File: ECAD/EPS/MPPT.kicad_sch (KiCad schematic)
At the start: 22 parts, among them U13 INA180A3, U14 INA180A3, U15 LM358, U16 LT3652EMSE

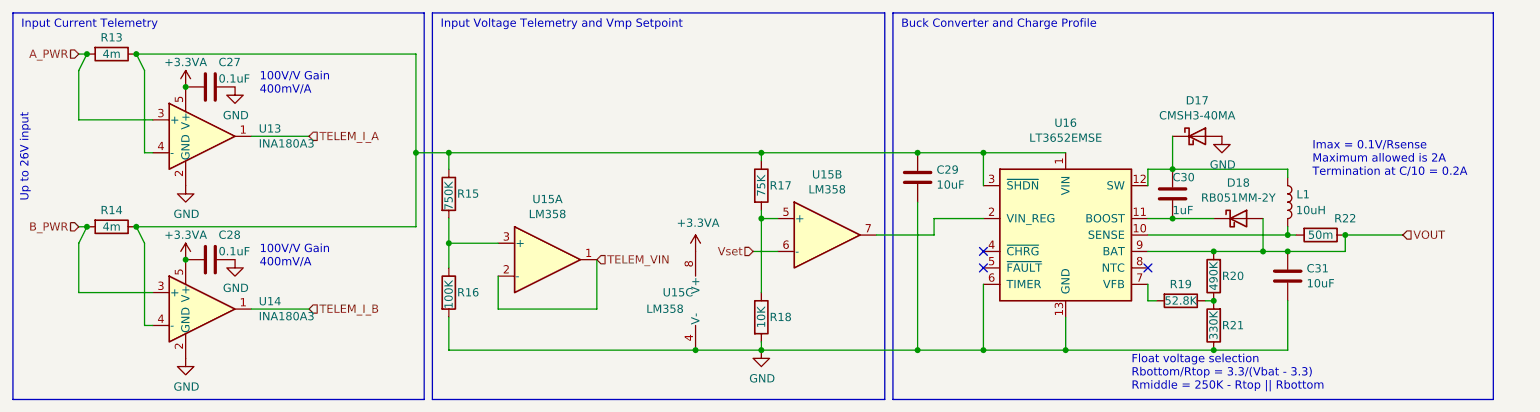
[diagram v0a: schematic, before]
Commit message: routing and stuff
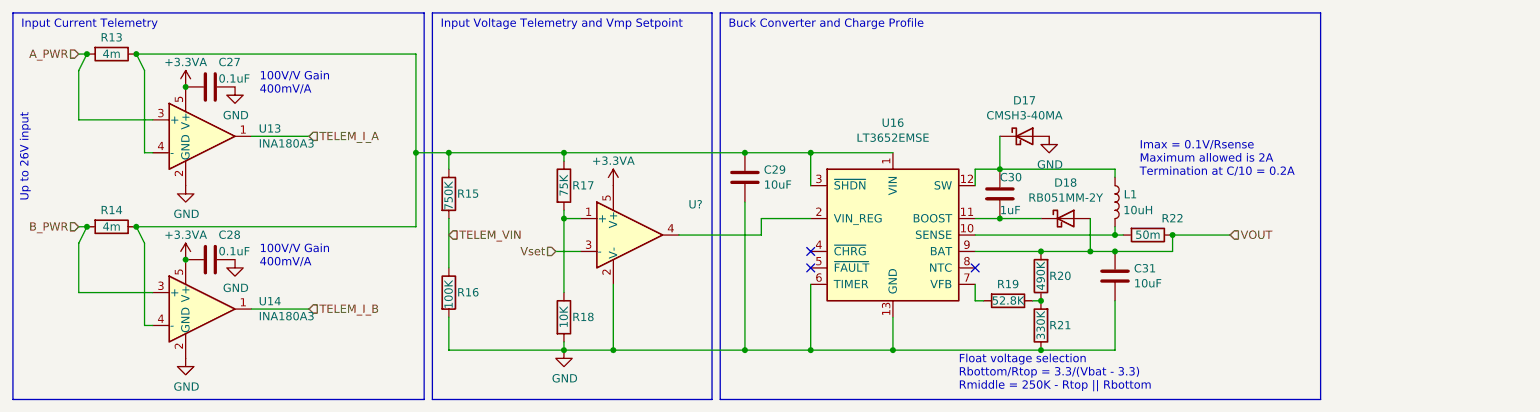
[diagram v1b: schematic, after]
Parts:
- removed U15: LM358, Package_SO:SO-8_3.9x4.9mm_P1.27mm, symbol Amplifier_Operational:LM358
- added U?: (no value), symbol Amplifier_Operational:LM321
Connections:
- net +3.3VA: now also U?.5 (V+)
- net GND: now also U?.2 (V-)
- net TELEM_VIN: now also R15.2, R16.1
- net Vset: now also U?.3 (-)
- net at U16.2 (VIN_REG): now also U?.4
- net at R17.2, R18.1: now also U?.1 (+)
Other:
- moved on the sheet: C29, C30, C31, D17, D18, L1, R17, R18, R19, R20, R21, R22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
